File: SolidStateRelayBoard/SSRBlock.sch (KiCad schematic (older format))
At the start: 8 parts, among them Q201 MMBT2222ALT1G, U201 SSR

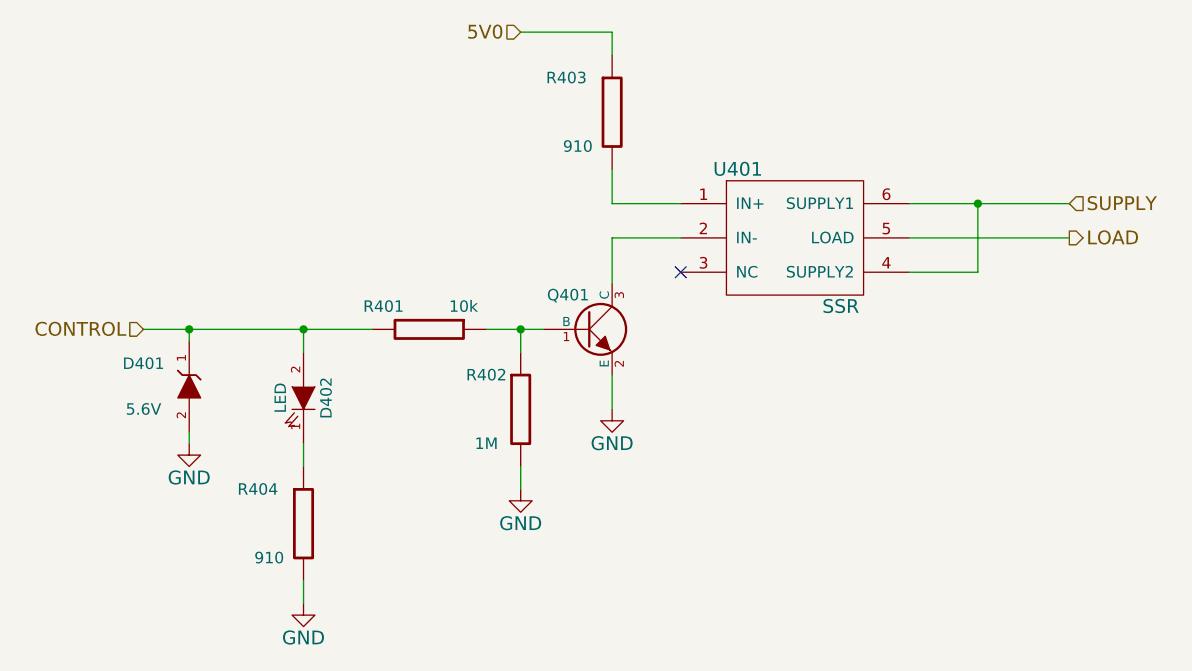
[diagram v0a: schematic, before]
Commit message: SSR Board
Small changes to PCB
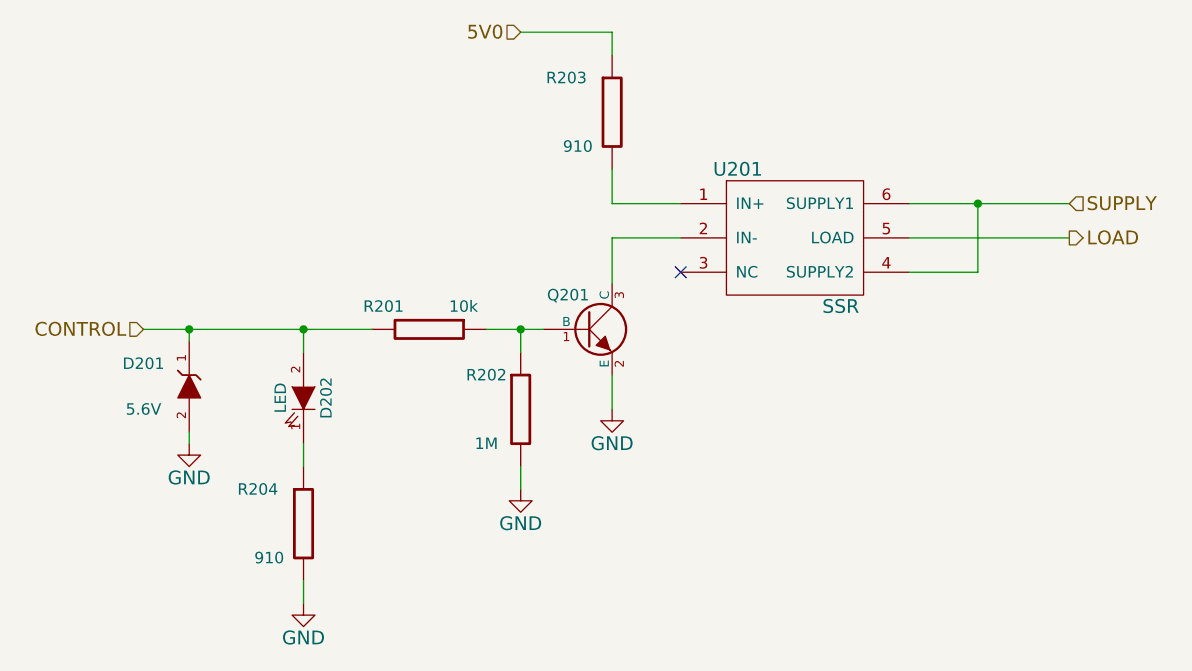
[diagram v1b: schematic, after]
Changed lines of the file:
@@
 $Descr A4 11693 8268
 encoding utf-8
-Sheet 4 14
+Sheet 2 14
 Title ""
 Date ""
@@
 AR Path="/586B7988/586B33BB" Ref="Q1601"  Part="1"
 AR Path="/586B7996/586B33BB" Ref="Q1701"  Part="1"
-F 0 "Q401" H 5100 3400 50  0000 R CNN
+F 0 "Q201" H 5100 3400 50  0000 R CNN
 F 1 "MMBT2222ALT1G" H 5100 3400 50  0001 R CNN
 F 2 "TO_SOT_Packages_SMD:SOT-23_Handsoldering" H 5100 3250 60  0001 C CNN
@@
 AR Path="/586B7988/586B33E9" Ref="R1603"  Part="1"
 AR Path="/586B7996/586B33E9" Ref="R1703"  Part="1"
-F 0 "R403" H 5000 2450 50  0000 C CNN
+F 0 "R203" H 5000 2450 50  0000 C CNN
 F 1 "910" H 5050 2150 50  0000 C CNN
 F 2 "Resistors_SMD:R_1206_HandSoldering" V 5130 2300 30  0001 C CNN
@@
 AR Path="/586B7988/586B3431" Ref="R1601"  Part="1"
 AR Path="/586B7996/586B3431" Ref="R1701"  Part="1"
-F 0 "R401" V 4300 3050 50  0000 C CNN
+F 0 "R201" V 4300 3050 50  0000 C CNN
 F 1 "10k" V 4300 3400 50  0000 C CNN
 F 2 "Resistors_SMD:R_1206_HandSoldering" V 4330 3250 30  0001 C CNN
@@
 	5200 3450 5200 3600
 $Comp
-L GND #PWR039
+L GND #PWR033
 U 1 1 586B354B
 P 5200 3600
-AR Path="/586B2B8E/586B354B" Ref="#PWR039"  Part="1"
-AR Path="/586B3F68/586B354B" Ref="#PWR043"  Part="1"
-AR Path="/586B4A2A/586B354B" Ref="#PWR047"  Part="1"
-AR Path="/586B4A38/586B354B" Ref="#PWR051"  Part="1"
-AR Path="/586B65A6/586B354B" Ref="#PWR055"  Part="1"
-AR Path="/586B65B4/586B354B" Ref="#PWR059"  Part="1"
-AR Path="/586B65C2/586B354B" Ref="#PWR063"  Part="1"
-AR Path="/586B65D0/586B354B" Ref="#PWR067"  Part="1"
-AR Path="/586B7934/586B354B" Ref="#PWR071"  Part="1"
-AR Path="/586B7942/586B354B" Ref="#PWR075"  Part="1"
-AR Path="/586B7950/586B354B" Ref="#PWR079"  Part="1"
-AR Path="/586B795E/586B354B" Ref="#PWR083"  Part="1"
-AR Path="/586B796C/586B354B" Ref="#PWR087"  Part="1"
+AR Path="/586B2B8E/586B354B" Ref="#PWR033"  Part="1"
+AR Path="/586B3F68/586B354B" Ref="#PWR037"  Part="1"
+AR Path="/586B4A2A/586B354B" Ref="#PWR041"  Part="1"
+AR Path="/586B4A38/586B354B" Ref="#PWR045"  Part="1"
+AR Path="/586B65A6/586B354B" Ref="#PWR049"  Part="1"
+AR Path="/586B65B4/586B354B" Ref="#PWR053"  Part="1"
+AR Path="/586B65C2/586B354B" Ref="#PWR057"  Part="1"
+AR Path="/586B65D0/586B354B" Ref="#PWR061"  Part="1"
+AR Path="/586B7934/586B354B" Ref="#PWR065"  Part="1"
+AR Path="/586B7942/586B354B" Ref="#PWR069"  Part="1"
+AR Path="/586B7950/586B354B" Ref="#PWR073"  Part="1"
+AR Path="/586B795E/586B354B" Ref="#PWR077"  Part="1"
+AR Path="/586B796C/586B354B" Ref="#PWR081"  Part="1"
 AR Path="/586B797A/586B354B" Ref="#PWR087"  Part="1"
 AR Path="/586B7988/586B354B" Ref="#PWR091"  Part="1"
 AR Path="/586B7996/586B354B" Ref="#PWR095"  Part="1"
-F 0 "#PWR087" H 5200 3350 60  0001 C CNN
+F 0 "#PWR033" H 5200 3350 60  0001 C CNN
 F 1 "GND" H 5200 3450 60  0000 C CNN
 F 2 "" H 5200 3600 60  0000 C CNN
@@
 AR Path="/586B7988/586B3681" Ref="D1601"  Part="1"
 AR Path="/586B7996/586B3681" Ref="D1701"  Part="1"
-F 0 "D401" V 3450 3700 50  0000 C CNN
+F 0 "D201" V 3450 3700 50  0000 C CNN
 F 1 "5.6V" V 3250 3700 50  0000 C CNN
 F 2 "hyperCustom:SOD-123" H 3350 3500 60  0001 C CNN
@@
 	3350 3700 3350 3750
 $Comp
-L GND #PWR040
+L GND #PWR034
 U 1 1 586B36D9
 P 3350 3750
-AR Path="/586B2B8E/586B36D9" Ref="#PWR040"  Part="1"
-AR Path="/586B3F68/586B36D9" Ref="#PWR044"  Part="1"
-AR Path="/586B4A2A/586B36D9" Ref="#PWR048"  Part="1"
-AR Path="/586B4A38/586B36D9" Ref="#PWR052"  Part="1"
-AR Path="/586B65A6/586B36D9" Ref="#PWR056"  Part="1"
-AR Path="/586B65B4/586B36D9" Ref="#PWR060"  Part="1"
-AR Path="/586B65C2/586B36D9" Ref="#PWR064"  Part="1"
-AR Path="/586B65D0/586B36D9" Ref="#PWR068"  Part="1"
-AR Path="/586B7934/586B36D9" Ref="#PWR072"  Part="1"
-AR Path="/586B7942/586B36D9" Ref="#PWR076"  Part="1"
-AR Path="/586B7950/586B36D9" Ref="#PWR080"  Part="1"
-AR Path="/586B795E/586B36D9" Ref="#PWR084"  Part="1"
-AR Path="/586B796C/586B36D9" Ref="#PWR088"  Part="1"
+AR Path="/586B2B8E/586B36D9" Ref="#PWR034"  Part="1"
+AR Path="/586B3F68/586B36D9" Ref="#PWR038"  Part="1"
+AR Path="/586B4A2A/586B36D9" Ref="#PWR042"  Part="1"
+AR Path="/586B4A38/586B36D9" Ref="#PWR046"  Part="1"
+AR Path="/586B65A6/586B36D9" Ref="#PWR050"  Part="1"
+AR Path="/586B65B4/586B36D9" Ref="#PWR054"  Part="1"
+AR Path="/586B65C2/586B36D9" Ref="#PWR058"  Part="1"
+AR Path="/586B65D0/586B36D9" Ref="#PWR062"  Part="1"
+AR Path="/586B7934/586B36D9" Ref="#PWR066"  Part="1"
+AR Path="/586B7942/586B36D9" Ref="#PWR070"  Part="1"
+AR Path="/586B7950/586B36D9" Ref="#PWR074"  Part="1"
+AR Path="/586B795E/586B36D9" Ref="#PWR078"  Part="1"
+AR Path="/586B796C/586B36D9" Ref="#PWR082"  Part="1"
 AR Path="/586B797A/586B36D9" Ref="#PWR088"  Part="1"
 AR Path="/586B7988/586B36D9" Ref="#PWR092"  Part="1"
 AR Path="/586B7996/586B36D9" Ref="#PWR096"  Part="1"
-F 0 "#PWR088" H 3350 3500 60  0001 C CNN
+F 0 "#PWR034" H 3350 3500 60  0001 C CNN
 F 1 "GND" H 3350 3600 60  0000 C CNN
 F 2 "" H 3350 3750 60  0000 C CNN
@@
 AR Path="/586B7988/586B39A4" Ref="R1602"  Part="1"
 AR Path="/586B7996/586B39A4" Ref="R1702"  Part="1"
-F 0 "R402" H 4650 3750 50  0000 C CNN
+F 0 "R202" H 4650 3750 50  0000 C CNN
 F 1 "1M" H 4650 3450 50  0000 C CNN
 F 2 "Resistors_SMD:R_1206_HandSoldering" V 4730 3600 30  0001 C CNN
@@
 	4800 3850 4800 3950
 $Comp
-L GND #PWR041
+L GND #PWR035
 U 1 1 586B3A19
 P 4800 3950
-AR Path="/586B2B8E/586B3A19" Ref="#PWR041"  Part="1"
-AR Path="/586B3F68/586B3A19" Ref="#PWR045"  Part="1"
-AR Path="/586B4A2A/586B3A19" Ref="#PWR049"  Part="1"
-AR Path="/586B4A38/586B3A19" Ref="#PWR053"  Part="1"
-AR Path="/586B65A6/586B3A19" Ref="#PWR057"  Part="1"
-AR Path="/586B65B4/586B3A19" Ref="#PWR061"  Part="1"
-AR Path="/586B65C2/586B3A19" Ref="#PWR065"  Part="1"
-AR Path="/586B65D0/586B3A19" Ref="#PWR069"  Part="1"
-AR Path="/586B7934/586B3A19" Ref="#PWR073"  Part="1"
-AR Path="/586B7942/586B3A19" Ref="#PWR077"  Part="1"
-AR Path="/586B7950/586B3A19" Ref="#PWR081"  Part="1"
-AR Path="/586B795E/586B3A19" Ref="#PWR085"  Part="1"
-AR Path="/586B796C/586B3A19" Ref="#PWR089"  Part="1"
+AR Path="/586B2B8E/586B3A19" Ref="#PWR035"  Part="1"
+AR Path="/586B3F68/586B3A19" Ref="#PWR039"  Part="1"
+AR Path="/586B4A2A/586B3A19" Ref="#PWR043"  Part="1"
+AR Path="/586B4A38/586B3A19" Ref="#PWR047"  Part="1"
+AR Path="/586B65A6/586B3A19" Ref="#PWR051"  Part="1"
+AR Path="/586B65B4/586B3A19" Ref="#PWR055"  Part="1"
+AR Path="/586B65C2/586B3A19" Ref="#PWR059"  Part="1"
+AR Path="/586B65D0/586B3A19" Ref="#PWR063"  Part="1"
+AR Path="/586B7934/586B3A19" Ref="#PWR067"  Part="1"
+AR Path="/586B7942/586B3A19" Ref="#PWR071"  Part="1"
+AR Path="/586B7950/586B3A19" Ref="#PWR075"  Part="1"
+AR Path="/586B795E/586B3A19" Ref="#PWR079"  Part="1"
+AR Path="/586B796C/586B3A19" Ref="#PWR083"  Part="1"
 AR Path="/586B797A/586B3A19" Ref="#PWR089"  Part="1"
 AR Path="/586B7988/586B3A19" Ref="#PWR093"  Part="1"
 AR Path="/586B7996/586B3A19" Ref="#PWR097"  Part="1"
-F 0 "#PWR089" H 4800 3700 60  0001 C CNN
+F 0 "#PWR035" H 4800 3700 60  0001 C CNN
 F 1 "GND" H 4800 3800 60  0000 C CNN
 F 2 "" H 4800 3950 60  0000 C CNN
@@
 AR Path="/586B7988/586D88E1" Ref="U1601"  Part="1"
 AR Path="/586B7996/586D88E1" Ref="U1701"  Part="1"
-F 0 "U401" H 5750 3150 60  0000 C CNN
+F 0 "U201" H 5750 3150 60  0000 C CNN
 F 1 "SSR" H 6200 2550 60  0000 C CNN
 F 2 "hyperCustom:VISHAY_6SMD_OPTOCOUPLER" H 6000 2850 60  0001 C CNN
@@
 AR Path="/586B7996/586E6B18" Ref="D1702"  Part="1"
 AR Path="/586E6B18" Ref="D202"  Part="1"
-F 0 "D402" H 3850 3650 50  0000 C CNN
+F 0 "D202" H 3850 3650 50  0000 C CNN
 F 1 "LED" H 3850 3450 50  0000 C CNN
 F 2 "hyperCustom:SOD-123" H 3850 3550 60  0001 C CNN
@@
 AR Path="/586B7988/586E6B5D" Ref="R1604"  Part="1"
 AR Path="/586B7996/586E6B5D" Ref="R1704"  Part="1"
-F 0 "R404" H 3650 4250 50  0000 C CNN
+F 0 "R204" H 3650 4250 50  0000 C CNN
 F 1 "910" H 3700 3950 50  0000 C CNN
 F 2 "Resistors_SMD:R_1206_HandSoldering" V 3780 4100 30  0001 C CNN
@@
 	3850 4350 3850 4450
 $Comp
-L GND #PWR042
+L GND #PWR036
 U 1 1 586E6C2B
 P 3850 4450
-AR Path="/586B2B8E/586E6C2B" Ref="#PWR042"  Part="1"
-AR Path="/586B3F68/586E6C2B" Ref="#PWR046"  Part="1"
-AR Path="/586B4A2A/586E6C2B" Ref="#PWR050"  Part="1"
-AR Path="/586B4A38/586E6C2B" Ref="#PWR054"  Part="1"
-AR Path="/586B65A6/586E6C2B" Ref="#PWR058"  Part="1"
-AR Path="/586B65B4/586E6C2B" Ref="#PWR062"  Part="1"
-AR Path="/586B65C2/586E6C2B" Ref="#PWR066"  Part="1"
-AR Path="/586B65D0/586E6C2B" Ref="#PWR070"  Part="1"
-AR Path="/586B7934/586E6C2B" Ref="#PWR074"  Part="1"
-AR Path="/586B7942/586E6C2B" Ref="#PWR078"  Part="1"
-AR Path="/586B7950/586E6C2B" Ref="#PWR082"  Part="1"
-AR Path="/586B795E/586E6C2B" Ref="#PWR086"  Part="1"
-AR Path="/586B796C/586E6C2B" Ref="#PWR090"  Part="1"
+AR Path="/586B2B8E/586E6C2B" Ref="#PWR036"  Part="1"
+AR Path="/586B3F68/586E6C2B" Ref="#PWR040"  Part="1"
+AR Path="/586B4A2A/586E6C2B" Ref="#PWR044"  Part="1"
+AR Path="/586B4A38/586E6C2B" Ref="#PWR048"  Part="1"
+AR Path="/586B65A6/586E6C2B" Ref="#PWR052"  Part="1"
+AR Path="/586B65B4/586E6C2B" Ref="#PWR056"  Part="1"
+AR Path="/586B65C2/586E6C2B" Ref="#PWR060"  Part="1"
+AR Path="/586B65D0/586E6C2B" Ref="#PWR064"  Part="1"
+AR Path="/586B7934/586E6C2B" Ref="#PWR068"  Part="1"
+AR Path="/586B7942/586E6C2B" Ref="#PWR072"  Part="1"
+AR Path="/586B7950/586E6C2B" Ref="#PWR076"  Part="1"
+AR Path="/586B795E/586E6C2B" Ref="#PWR080"  Part="1"
+AR Path="/586B796C/586E6C2B" Ref="#PWR084"  Part="1"
 AR Path="/586B797A/586E6C2B" Ref="#PWR090"  Part="1"
 AR Path="/586B7988/586E6C2B" Ref="#PWR094"  Part="1"
 AR Path="/586B7996/586E6C2B" Ref="#PWR098"  Part="1"
-F 0 "#PWR090" H 3850 4200 60  0001 C CNN
+F 0 "#PWR036" H 3850 4200 60  0001 C CNN
 F 1 "GND" H 3850 4300 60  0000 C CNN
 F 2 "" H 3850 4450 60  0000 C CNN
